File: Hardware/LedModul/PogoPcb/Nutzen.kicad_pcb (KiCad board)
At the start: 2 copper layers, 96 x 96 mm, 150 parts, among them J1 Conn_01x01_Pin, J2 Conn_01x01_Pin, J3 Conn_01x01_Pin, J4 Conn_01x01_Pin, J5 Conn_01x01_Pin, J6 Conn_01x01_Pin

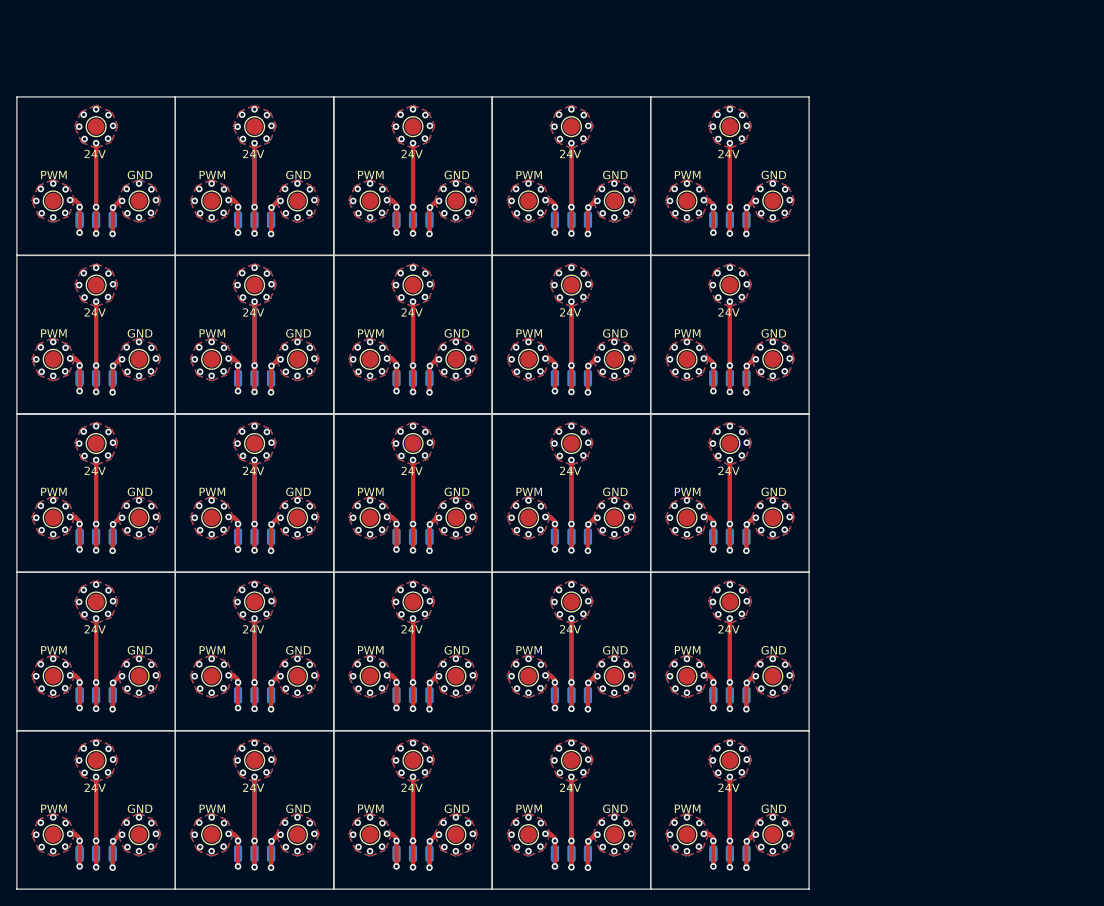
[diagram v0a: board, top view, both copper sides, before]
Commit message: added gerber data
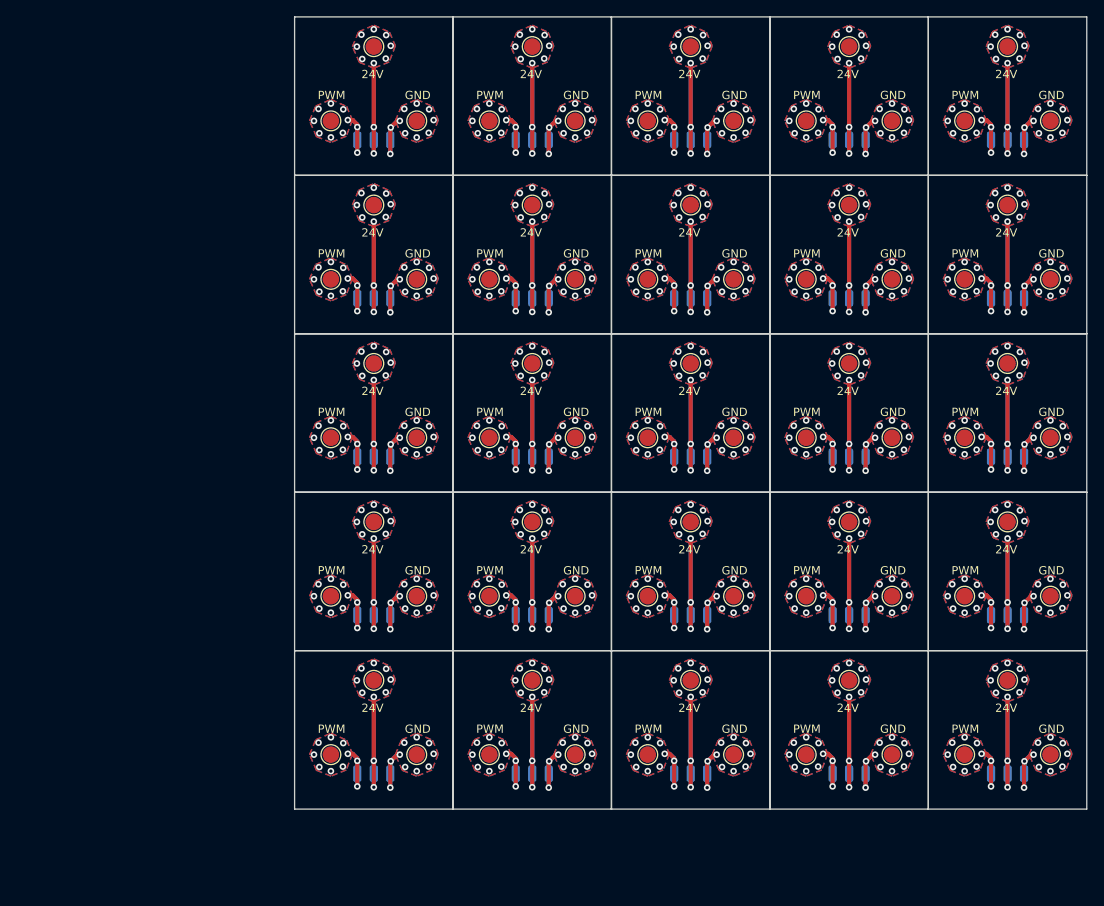
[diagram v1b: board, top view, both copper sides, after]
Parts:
- removed the J1 at (80.4, 98.5)
- removed the J1 at (99.6, 79.3)
- removed the J1 at (157.2, 79.3)
- removed the J1 at (138.0, 79.3)
- removed the J1 at (99.6, 60.1)
- removed the J1 at (138.0, 98.5)
- removed the J1 at (80.4, 79.3)
- removed the J1 at (118.8, 60.1)
- removed the J1 at (138.0, 136.9)
- removed the J1 at (99.6, 136.9)
- removed the J1 at (157.2, 60.1)
- removed the J1 at (99.6, 117.7)
- removed the J1 at (138.0, 60.1)
- removed the J1 at (118.8, 79.3)
- removed the J1 at (99.6, 98.5)
- removed the J1 at (80.4, 136.9)
- removed the J1 at (157.2, 117.7)
- removed the J1 at (138.0, 117.7)
- removed the J1 at (157.2, 136.9)
- removed the J1 at (80.4, 117.7)
- removed the J1 at (157.2, 98.5)
- removed the J1 at (118.8, 117.7)
- removed the J1 at (80.4, 60.1)
- removed the J1 at (118.8, 136.9)
- removed the J1 at (118.8, 98.5)
- removed the J2 at (102.8, 115.4)
- removed the J2 at (122.0, 115.4)
- removed the J2 at (83.6, 115.4)
- removed the J2 at (160.4, 134.6)
- removed the J2 at (160.4, 57.8)
- removed the J2 at (102.8, 96.2)
- removed the J2 at (102.8, 134.6)
- removed the J2 at (141.2, 134.6)
- removed the J2 at (141.2, 57.8)
- removed the J2 at (102.8, 57.8)
- removed the J2 at (141.2, 115.4)
- removed the J2 at (102.8, 77.0)
- removed the J2 at (122.0, 96.2)
- removed the J2 at (83.6, 77.0)
- removed the J2 at (141.2, 77.0)
- removed the J2 at (160.4, 96.2)
- removed the J2 at (122.0, 57.8)
- removed the J2 at (141.2, 96.2)
- removed the J2 at (122.0, 77.0)
- removed the J2 at (160.4, 115.4)
- removed the J2 at (122.0, 134.6)
- removed the J2 at (160.4, 77.0)
- removed the J2 at (83.6, 96.2)
- removed the J2 at (83.6, 134.6)
- removed the J2 at (83.6, 57.8)
- removed the J3 at (73.2, 77.0)
- removed the J3 at (73.2, 134.6)
- removed the J3 at (92.4, 77.0)
- removed the J3 at (92.4, 57.8)
- removed the J3 at (73.2, 57.8)
- removed the J3 at (150.0, 96.2)
- removed the J3 at (73.2, 96.2)
- removed the J3 at (130.8, 77.0)
- removed the J3 at (130.8, 57.8)
- removed the J3 at (111.6, 115.4)
- removed the J3 at (92.4, 96.2)
- removed the J3 at (111.6, 96.2)
- removed the J3 at (111.6, 134.6)
- removed the J3 at (130.8, 134.6)
- removed the J3 at (111.6, 57.8)
- removed the J3 at (150.0, 134.6)
- removed the J3 at (73.2, 115.4)
- removed the J3 at (150.0, 77.0)
- removed the J3 at (111.6, 77.0)
- removed the J3 at (150.0, 57.8)
- removed the J3 at (92.4, 134.6)
- removed the J3 at (92.4, 115.4)
- removed the J3 at (150.0, 115.4)
- removed the J3 at (130.8, 115.4)
- removed the J3 at (130.8, 96.2)
- removed the J4 at (134.0, 117.7)
- removed the J4 at (114.8, 98.5)
- removed the J4 at (114.8, 136.9)
- removed the J4 at (114.8, 117.7)
- removed the J4 at (76.4, 98.5)
- removed the J4 at (95.6, 98.5)
- removed the J4 at (76.4, 136.9)
- removed the J4 at (153.2, 60.1)
- removed the J4 at (114.8, 79.3)
- removed the J4 at (114.8, 60.1)
- removed the J4 at (76.4, 60.1)
- removed the J4 at (95.6, 136.9)
- removed the J4 at (134.0, 98.5)
- removed the J4 at (95.6, 79.3)
- removed the J4 at (134.0, 136.9)
- removed the J4 at (153.2, 98.5)
- removed the J4 at (95.6, 60.1)
- removed the J4 at (153.2, 136.9)
- removed the J4 at (134.0, 79.3)
- removed the J4 at (76.4, 79.3)
- removed the J4 at (95.6, 117.7)
- removed the J4 at (76.4, 117.7)
- removed the J4 at (134.0, 60.1)
- removed the J4 at (153.2, 117.7)
- removed the J4 at (153.2, 79.3)
- removed the J5 at (155.2, 68.0)
- removed the J5 at (78.4, 106.4)
- removed the J5 at (97.6, 87.2)
- removed the J5 at (78.4, 68.0)
- removed the J5 at (136.0, 87.2)
- removed the J5 at (136.0, 48.8)
- removed the J5 at (155.2, 125.6)
- removed the J5 at (116.8, 106.4)
- removed the J5 at (155.2, 48.8)
- removed the J5 at (116.8, 68.0)
- removed the J5 at (116.8, 125.6)
- removed the J5 at (97.6, 125.6)
- removed the J5 at (116.8, 87.2)
- removed the J5 at (136.0, 125.6)
- removed the J5 at (97.6, 106.4)
- removed the J5 at (78.4, 48.8)
- removed the J5 at (136.0, 68.0)
- removed the J5 at (78.4, 87.2)
- removed the J5 at (97.6, 68.0)
- removed the J5 at (155.2, 106.4)
- removed the J5 at (136.0, 106.4)
- removed the J5 at (155.2, 87.2)
- removed the J5 at (116.8, 48.8)
- removed the J5 at (97.6, 48.8)
- removed the J5 at (78.4, 125.6)
- removed the J6 at (97.6, 136.9)
- removed the J6 at (97.6, 60.1)
- removed the J6 at (116.8, 79.3)
- removed the J6 at (155.2, 117.7)
- removed the J6 at (78.4, 98.5)
- removed the J6 at (78.4, 79.3)
- removed the J6 at (78.4, 117.7)
- removed the J6 at (136.0, 79.3)
- removed the J6 at (97.6, 98.5)
- removed the J6 at (116.8, 98.5)
- removed the J6 at (155.2, 79.3)
- removed the J6 at (136.0, 136.9)
- removed the J6 at (136.0, 60.1)
- removed the J6 at (97.6, 117.7)
- removed the J6 at (78.4, 60.1)
- removed the J6 at (97.6, 79.3)
- removed the J6 at (155.2, 60.1)
- removed the J6 at (116.8, 117.7)
- removed the J6 at (155.2, 98.5)
- removed the J6 at (155.2, 136.9)
- removed the J6 at (78.4, 136.9)
- removed the J6 at (116.8, 136.9)
- removed the J6 at (136.0, 98.5)
- removed the J6 at (136.0, 117.7)
- removed the J6 at (116.8, 60.1)
- added J1: Conn_01x01_Pin, Bergi:Solderpad_1x2, B.Cu at (114.0, 88.8)
- added J1: Conn_01x01_Pin, Bergi:Solderpad_1x2, B.Cu at (190.8, 88.8)
- added J1: Conn_01x01_Pin, Bergi:Solderpad_1x2, B.Cu at (171.7, 108.0)
- added J1: Conn_01x01_Pin, Bergi:Solderpad_1x2, B.Cu at (133.2, 50.4)
- added J1: Conn_01x01_Pin, Bergi:Solderpad_1x2, B.Cu at (133.2, 127.2)
- added J1: Conn_01x01_Pin, Bergi:Solderpad_1x2, B.Cu at (190.8, 50.4)
- added J1: Conn_01x01_Pin, Bergi:Solderpad_1x2, B.Cu at (171.7, 50.4)
- added J1: Conn_01x01_Pin, Bergi:Solderpad_1x2, B.Cu at (152.4, 88.8)
- added J1: Conn_01x01_Pin, Bergi:Solderpad_1x2, B.Cu at (114.0, 69.6)
- added J1: Conn_01x01_Pin, Bergi:Solderpad_1x2, B.Cu at (190.8, 127.2)
- added J1: Conn_01x01_Pin, Bergi:Solderpad_1x2, B.Cu at (152.4, 127.2)
- added J1: Conn_01x01_Pin, Bergi:Solderpad_1x2, B.Cu at (133.2, 108.0)
- added J1: Conn_01x01_Pin, Bergi:Solderpad_1x2, B.Cu at (114.0, 127.2)
- added J1: Conn_01x01_Pin, Bergi:Solderpad_1x2, B.Cu at (114.0, 108.0)
- added J1: Conn_01x01_Pin, Bergi:Solderpad_1x2, B.Cu at (152.4, 50.4)
- added J1: Conn_01x01_Pin, Bergi:Solderpad_1x2, B.Cu at (133.2, 88.8)
- added J1: Conn_01x01_Pin, Bergi:Solderpad_1x2, B.Cu at (171.7, 127.2)
- added J1: Conn_01x01_Pin, Bergi:Solderpad_1x2, B.Cu at (152.4, 108.0)
- added J1: Conn_01x01_Pin, Bergi:Solderpad_1x2, B.Cu at (171.7, 88.8)
- added J1: Conn_01x01_Pin, Bergi:Solderpad_1x2, B.Cu at (171.7, 69.6)
- added J1: Conn_01x01_Pin, Bergi:Solderpad_1x2, B.Cu at (133.2, 69.6)
- added J1: Conn_01x01_Pin, Bergi:Solderpad_1x2, B.Cu at (114.0, 50.4)
- added J1: Conn_01x01_Pin, Bergi:Solderpad_1x2, B.Cu at (152.4, 69.6)
- added J1: Conn_01x01_Pin, Bergi:Solderpad_1x2, B.Cu at (190.8, 108.0)
- added J1: Conn_01x01_Pin, Bergi:Solderpad_1x2, B.Cu at (190.8, 69.6)
- added J2: Conn_01x01_Pin, TestPoint:TestPoint_Pad_D2.0mm, F.Cu at (136.4, 67.3)
- added J2: Conn_01x01_Pin, TestPoint:TestPoint_Pad_D2.0mm, F.Cu at (194.1, 48.1)
- added J2: Conn_01x01_Pin, TestPoint:TestPoint_Pad_D2.0mm, F.Cu at (194.1, 86.5)
- added J2: Conn_01x01_Pin, TestPoint:TestPoint_Pad_D2.0mm, F.Cu at (155.7, 48.1)
- added J2: Conn_01x01_Pin, TestPoint:TestPoint_Pad_D2.0mm, F.Cu at (117.2, 67.3)
- added J2: Conn_01x01_Pin, TestPoint:TestPoint_Pad_D2.0mm, F.Cu at (155.7, 86.5)
- added J2: Conn_01x01_Pin, TestPoint:TestPoint_Pad_D2.0mm, F.Cu at (174.8, 86.5)
- added J2: Conn_01x01_Pin, TestPoint:TestPoint_Pad_D2.0mm, F.Cu at (155.7, 105.7)
- added J2: Conn_01x01_Pin, TestPoint:TestPoint_Pad_D2.0mm, F.Cu at (155.7, 67.3)
- added J2: Conn_01x01_Pin, TestPoint:TestPoint_Pad_D2.0mm, F.Cu at (194.1, 105.7)
- added J2: Conn_01x01_Pin, TestPoint:TestPoint_Pad_D2.0mm, F.Cu at (117.2, 124.9)
- added J2: Conn_01x01_Pin, TestPoint:TestPoint_Pad_D2.0mm, F.Cu at (136.4, 86.5)
- added J2: Conn_01x01_Pin, TestPoint:TestPoint_Pad_D2.0mm, F.Cu at (117.2, 105.7)
- added J2: Conn_01x01_Pin, TestPoint:TestPoint_Pad_D2.0mm, F.Cu at (117.2, 48.1)
- added J2: Conn_01x01_Pin, TestPoint:TestPoint_Pad_D2.0mm, F.Cu at (194.1, 124.9)
- added J2: Conn_01x01_Pin, TestPoint:TestPoint_Pad_D2.0mm, F.Cu at (136.4, 48.1)
- added J2: Conn_01x01_Pin, TestPoint:TestPoint_Pad_D2.0mm, F.Cu at (174.8, 67.3)
- added J2: Conn_01x01_Pin, TestPoint:TestPoint_Pad_D2.0mm, F.Cu at (136.4, 124.9)
- added J2: Conn_01x01_Pin, TestPoint:TestPoint_Pad_D2.0mm, F.Cu at (117.2, 86.5)
- added J2: Conn_01x01_Pin, TestPoint:TestPoint_Pad_D2.0mm, F.Cu at (155.7, 124.9)
- added J2: Conn_01x01_Pin, TestPoint:TestPoint_Pad_D2.0mm, F.Cu at (174.8, 105.7)
- added J2: Conn_01x01_Pin, TestPoint:TestPoint_Pad_D2.0mm, F.Cu at (136.4, 105.7)
- added J2: Conn_01x01_Pin, TestPoint:TestPoint_Pad_D2.0mm, F.Cu at (174.8, 124.9)
- added J2: Conn_01x01_Pin, TestPoint:TestPoint_Pad_D2.0mm, F.Cu at (194.1, 67.3)
- added J2: Conn_01x01_Pin, TestPoint:TestPoint_Pad_D2.0mm, F.Cu at (174.8, 48.1)
- added J3: Conn_01x01_Pin, TestPoint:TestPoint_Pad_D2.0mm, F.Cu at (126.0, 48.1)
- added J3: Conn_01x01_Pin, TestPoint:TestPoint_Pad_D2.0mm, F.Cu at (126.0, 105.7)
- added J3: Conn_01x01_Pin, TestPoint:TestPoint_Pad_D2.0mm, F.Cu at (164.4, 86.5)
- added J3: Conn_01x01_Pin, TestPoint:TestPoint_Pad_D2.0mm, F.Cu at (183.7, 86.5)
- added J3: Conn_01x01_Pin, TestPoint:TestPoint_Pad_D2.0mm, F.Cu at (164.4, 48.1)
- added J3: Conn_01x01_Pin, TestPoint:TestPoint_Pad_D2.0mm, F.Cu at (164.4, 105.7)
- added J3: Conn_01x01_Pin, TestPoint:TestPoint_Pad_D2.0mm, F.Cu at (145.2, 124.9)
- added J3: Conn_01x01_Pin, TestPoint:TestPoint_Pad_D2.0mm, F.Cu at (183.7, 105.7)
- added J3: Conn_01x01_Pin, TestPoint:TestPoint_Pad_D2.0mm, F.Cu at (145.2, 105.7)
- added J3: Conn_01x01_Pin, TestPoint:TestPoint_Pad_D2.0mm, F.Cu at (126.0, 124.9)
- added J3: Conn_01x01_Pin, TestPoint:TestPoint_Pad_D2.0mm, F.Cu at (183.7, 124.9)
- added J3: Conn_01x01_Pin, TestPoint:TestPoint_Pad_D2.0mm, F.Cu at (183.7, 67.3)
- added J3: Conn_01x01_Pin, TestPoint:TestPoint_Pad_D2.0mm, F.Cu at (106.8, 124.9)
- added J3: Conn_01x01_Pin, TestPoint:TestPoint_Pad_D2.0mm, F.Cu at (145.2, 48.1)
- added J3: Conn_01x01_Pin, TestPoint:TestPoint_Pad_D2.0mm, F.Cu at (106.8, 48.1)
- added J3: Conn_01x01_Pin, TestPoint:TestPoint_Pad_D2.0mm, F.Cu at (145.2, 67.3)
- added J3: Conn_01x01_Pin, TestPoint:TestPoint_Pad_D2.0mm, F.Cu at (106.8, 86.5)
- added J3: Conn_01x01_Pin, TestPoint:TestPoint_Pad_D2.0mm, F.Cu at (106.8, 67.3)
- added J3: Conn_01x01_Pin, TestPoint:TestPoint_Pad_D2.0mm, F.Cu at (145.2, 86.5)
- added J3: Conn_01x01_Pin, TestPoint:TestPoint_Pad_D2.0mm, F.Cu at (164.4, 124.9)
- added J3: Conn_01x01_Pin, TestPoint:TestPoint_Pad_D2.0mm, F.Cu at (164.4, 67.3)
- added J3: Conn_01x01_Pin, TestPoint:TestPoint_Pad_D2.0mm, F.Cu at (183.7, 48.1)
- added J3: Conn_01x01_Pin, TestPoint:TestPoint_Pad_D2.0mm, F.Cu at (126.0, 86.5)
- added J3: Conn_01x01_Pin, TestPoint:TestPoint_Pad_D2.0mm, F.Cu at (126.0, 67.3)
- added J3: Conn_01x01_Pin, TestPoint:TestPoint_Pad_D2.0mm, F.Cu at (106.8, 105.7)
- added J4: Conn_01x01_Pin, Bergi:Solderpad_1x2, B.Cu at (167.7, 108.0)
- added J4: Conn_01x01_Pin, Bergi:Solderpad_1x2, B.Cu at (167.7, 127.2)
- added J4: Conn_01x01_Pin, Bergi:Solderpad_1x2, B.Cu at (110.0, 108.0)
- added J4: Conn_01x01_Pin, Bergi:Solderpad_1x2, B.Cu at (148.4, 88.8)
- added J4: Conn_01x01_Pin, Bergi:Solderpad_1x2, B.Cu at (186.8, 88.8)
- added J4: Conn_01x01_Pin, Bergi:Solderpad_1x2, B.Cu at (186.8, 108.0)
- added J4: Conn_01x01_Pin, Bergi:Solderpad_1x2, B.Cu at (129.2, 50.4)
- added J4: Conn_01x01_Pin, Bergi:Solderpad_1x2, B.Cu at (129.2, 127.2)
- added J4: Conn_01x01_Pin, Bergi:Solderpad_1x2, B.Cu at (129.2, 69.6)
- added J4: Conn_01x01_Pin, Bergi:Solderpad_1x2, B.Cu at (129.2, 108.0)
- added J4: Conn_01x01_Pin, Bergi:Solderpad_1x2, B.Cu at (148.4, 50.4)
- added J4: Conn_01x01_Pin, Bergi:Solderpad_1x2, B.Cu at (167.7, 88.8)
- added J4: Conn_01x01_Pin, Bergi:Solderpad_1x2, B.Cu at (167.7, 69.6)
- added J4: Conn_01x01_Pin, Bergi:Solderpad_1x2, B.Cu at (129.2, 88.8)
- added J4: Conn_01x01_Pin, Bergi:Solderpad_1x2, B.Cu at (110.0, 88.8)
- added J4: Conn_01x01_Pin, Bergi:Solderpad_1x2, B.Cu at (186.8, 50.4)
- added J4: Conn_01x01_Pin, Bergi:Solderpad_1x2, B.Cu at (186.8, 69.6)
- added J4: Conn_01x01_Pin, Bergi:Solderpad_1x2, B.Cu at (167.7, 50.4)
- added J4: Conn_01x01_Pin, Bergi:Solderpad_1x2, B.Cu at (148.4, 108.0)
- added J4: Conn_01x01_Pin, Bergi:Solderpad_1x2, B.Cu at (110.0, 127.2)
- added J4: Conn_01x01_Pin, Bergi:Solderpad_1x2, B.Cu at (148.4, 127.2)
- added J4: Conn_01x01_Pin, Bergi:Solderpad_1x2, B.Cu at (186.8, 127.2)
- added J4: Conn_01x01_Pin, Bergi:Solderpad_1x2, B.Cu at (110.0, 50.4)
- added J4: Conn_01x01_Pin, Bergi:Solderpad_1x2, B.Cu at (110.0, 69.6)
- added J4: Conn_01x01_Pin, Bergi:Solderpad_1x2, B.Cu at (148.4, 69.6)
- added J5: Conn_01x01_Pin, TestPoint:TestPoint_Pad_D2.0mm, F.Cu at (131.2, 115.9)
- added J5: Conn_01x01_Pin, TestPoint:TestPoint_Pad_D2.0mm, F.Cu at (112.0, 96.7)
- added J5: Conn_01x01_Pin, TestPoint:TestPoint_Pad_D2.0mm, F.Cu at (112.0, 58.3)
- added J5: Conn_01x01_Pin, TestPoint:TestPoint_Pad_D2.0mm, F.Cu at (112.0, 39.1)
- added J5: Conn_01x01_Pin, TestPoint:TestPoint_Pad_D2.0mm, F.Cu at (131.2, 77.5)
- added J5: Conn_01x01_Pin, TestPoint:TestPoint_Pad_D2.0mm, F.Cu at (188.8, 96.7)
- added J5: Conn_01x01_Pin, TestPoint:TestPoint_Pad_D2.0mm, F.Cu at (169.7, 115.9)
- added J5: Conn_01x01_Pin, TestPoint:TestPoint_Pad_D2.0mm, F.Cu at (169.7, 39.1)
- added J5: Conn_01x01_Pin, TestPoint:TestPoint_Pad_D2.0mm, F.Cu at (150.4, 96.7)
- added J5: Conn_01x01_Pin, TestPoint:TestPoint_Pad_D2.0mm, F.Cu at (112.0, 115.9)
- added J5: Conn_01x01_Pin, TestPoint:TestPoint_Pad_D2.0mm, F.Cu at (112.0, 77.5)
- added J5: Conn_01x01_Pin, TestPoint:TestPoint_Pad_D2.0mm, F.Cu at (131.2, 58.3)
- added J5: Conn_01x01_Pin, TestPoint:TestPoint_Pad_D2.0mm, F.Cu at (188.8, 115.9)
- added J5: Conn_01x01_Pin, TestPoint:TestPoint_Pad_D2.0mm, F.Cu at (131.2, 96.7)
- added J5: Conn_01x01_Pin, TestPoint:TestPoint_Pad_D2.0mm, F.Cu at (169.7, 58.3)
- added J5: Conn_01x01_Pin, TestPoint:TestPoint_Pad_D2.0mm, F.Cu at (169.7, 77.5)
- added J5: Conn_01x01_Pin, TestPoint:TestPoint_Pad_D2.0mm, F.Cu at (188.8, 77.5)
- added J5: Conn_01x01_Pin, TestPoint:TestPoint_Pad_D2.0mm, F.Cu at (150.4, 77.5)
- added J5: Conn_01x01_Pin, TestPoint:TestPoint_Pad_D2.0mm, F.Cu at (188.8, 39.1)
- added J5: Conn_01x01_Pin, TestPoint:TestPoint_Pad_D2.0mm, F.Cu at (131.2, 39.1)
- added J5: Conn_01x01_Pin, TestPoint:TestPoint_Pad_D2.0mm, F.Cu at (169.7, 96.7)
- added J5: Conn_01x01_Pin, TestPoint:TestPoint_Pad_D2.0mm, F.Cu at (188.8, 58.3)
- added J5: Conn_01x01_Pin, TestPoint:TestPoint_Pad_D2.0mm, F.Cu at (150.4, 115.9)
- added J5: Conn_01x01_Pin, TestPoint:TestPoint_Pad_D2.0mm, F.Cu at (150.4, 39.1)
- added J5: Conn_01x01_Pin, TestPoint:TestPoint_Pad_D2.0mm, F.Cu at (150.4, 58.3)
- added J6: Conn_01x01_Pin, Bergi:Solderpad_1x2, B.Cu at (169.7, 127.2)
- added J6: Conn_01x01_Pin, Bergi:Solderpad_1x2, B.Cu at (131.2, 127.2)
- added J6: Conn_01x01_Pin, Bergi:Solderpad_1x2, B.Cu at (112.0, 69.6)
- added J6: Conn_01x01_Pin, Bergi:Solderpad_1x2, B.Cu at (131.2, 88.8)
- added J6: Conn_01x01_Pin, Bergi:Solderpad_1x2, B.Cu at (188.8, 88.8)
- added J6: Conn_01x01_Pin, Bergi:Solderpad_1x2, B.Cu at (150.4, 50.4)
- added J6: Conn_01x01_Pin, Bergi:Solderpad_1x2, B.Cu at (131.2, 50.4)
- added J6: Conn_01x01_Pin, Bergi:Solderpad_1x2, B.Cu at (150.4, 108.0)
- added J6: Conn_01x01_Pin, Bergi:Solderpad_1x2, B.Cu at (112.0, 108.0)
- added J6: Conn_01x01_Pin, Bergi:Solderpad_1x2, B.Cu at (169.7, 50.4)
- added J6: Conn_01x01_Pin, Bergi:Solderpad_1x2, B.Cu at (150.4, 88.8)
- added J6: Conn_01x01_Pin, Bergi:Solderpad_1x2, B.Cu at (150.4, 127.2)
- added J6: Conn_01x01_Pin, Bergi:Solderpad_1x2, B.Cu at (169.7, 69.6)
- added J6: Conn_01x01_Pin, Bergi:Solderpad_1x2, B.Cu at (112.0, 127.2)
- added J6: Conn_01x01_Pin, Bergi:Solderpad_1x2, B.Cu at (169.7, 108.0)
- added J6: Conn_01x01_Pin, Bergi:Solderpad_1x2, B.Cu at (131.2, 108.0)
- added J6: Conn_01x01_Pin, Bergi:Solderpad_1x2, B.Cu at (188.8, 108.0)
- added J6: Conn_01x01_Pin, Bergi:Solderpad_1x2, B.Cu at (150.4, 69.6)
- added J6: Conn_01x01_Pin, Bergi:Solderpad_1x2, B.Cu at (112.0, 50.4)
- added J6: Conn_01x01_Pin, Bergi:Solderpad_1x2, B.Cu at (188.8, 69.6)
- added J6: Conn_01x01_Pin, Bergi:Solderpad_1x2, B.Cu at (169.7, 88.8)
- added J6: Conn_01x01_Pin, Bergi:Solderpad_1x2, B.Cu at (112.0, 88.8)
- added J6: Conn_01x01_Pin, Bergi:Solderpad_1x2, B.Cu at (188.8, 127.2)
- added J6: Conn_01x01_Pin, Bergi:Solderpad_1x2, B.Cu at (131.2, 69.6)
- added J6: Conn_01x01_Pin, Bergi:Solderpad_1x2, B.Cu at (188.8, 50.4)
